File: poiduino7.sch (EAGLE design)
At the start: 20 parts, among them K1 TS-1109, Y1 16MHZ

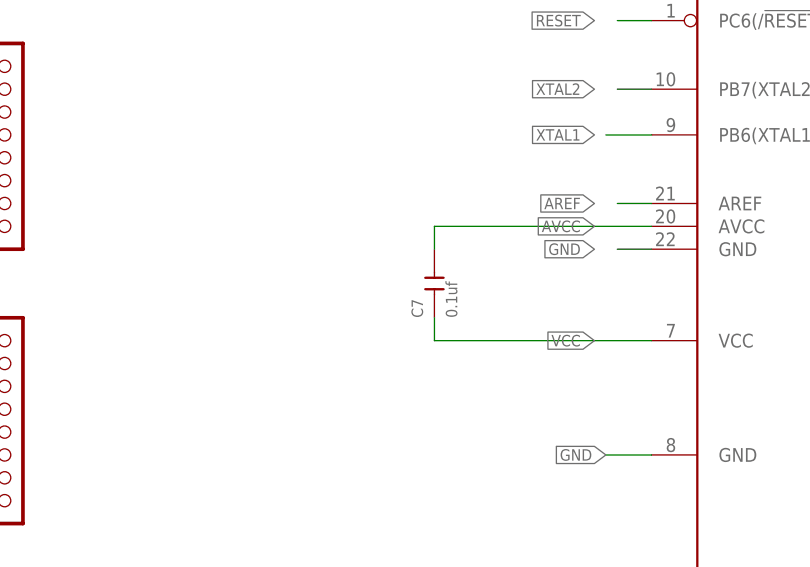
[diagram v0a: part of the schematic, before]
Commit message: new board
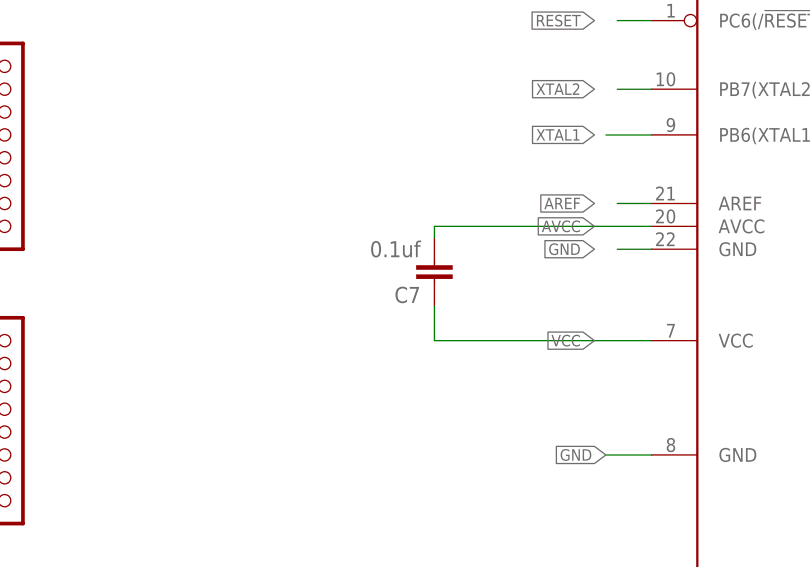
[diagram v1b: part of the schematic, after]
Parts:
- C7: device Seeed-Capacitor:DIP-CERAMIC-DISC-10NF-50V-Y5V(D4.0MM) -> capacitor-wima:C5/2.5
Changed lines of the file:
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@@
 <?xml version="1.0" encoding="utf-8"?>
 <!DOCTYPE eagle SYSTEM "eagle.dtd">
-<eagle version="7.7.0">
+<eagle version="9.0.0">
 <drawing>
 <settings>
 <setting alwaysvectorfont="no"/>
+<setting keepoldvectorfont="yes"/>
 <setting verticaltext="up"/>
 </settings>
-<grid distance="0.05" unitdist="inch" unit="inch" style="lines" multiple="1" display="yes" altdistance="0.001" altunitdist="inch" altunit="inch"/>
+<grid distance="0.1" unitdist="inch" unit="inch" style="lines" multiple="1" display="no" altdistance="0.01" altunitdist="inch" altunit="inch"/>
 <layers>
 <layer number="1" name="Top" color="4" fill="1" visible="no" active="no"/>
@@
 <part name="D1" library="Seeed-LED" deviceset="DIP-LED-GREEN-GREEN(2P-D3MM)" device="" value="CX-G302DC"/>
 <part name="D2" library="Seeed-LED" deviceset="DIP-LED-GREEN-GREEN(2P-D3MM)" device="" value="CX-G302DC"/>
-<part name="U1" library="Seeed-IC" deviceset="MCU-ATMEGA328P-PU(DIP28)" device=""/>
+<part name="U1" library="Seeed-IC" library_urn="urn:adsk.eagle:library:470" deviceset="MCU-ATMEGA328P-PU(DIP28)" device="" package3d_urn="urn:adsk.eagle:package:32652/1"/>
 <part name="Y1" library="Seeed-Crystal Oscillator" deviceset="DIP-CRYSTAL-16MHZ-18PF-30PPM-40R(HC49US)" device="" value="16MHZ"/>
 <part name="R1" library="Seeed-Resistor" deviceset="DIP-RES-10K-5%-1/4W(PR-D2.3XL6.5MM)" device="" value="10K"/>
@@
 <part name="SUPPLY7" library="supply2" deviceset="GND" device=""/>
 <part name="P+3" library="supply1" deviceset="VCC" device=""/>
-<part name="C7" library="Seeed-Capacitor" deviceset="DIP-CERAMIC-DISC-10NF-50V-Y5V(D4.0MM)" device="" value="0.1uf"/>
+<part name="C7" library="capacitor-wima" library_urn="urn:adsk.eagle:library:116" deviceset="C" device="5/2.5" package3d_urn="urn:adsk.eagle:package:5426/1" value="0.1uf"/>
 </parts>
 <sheets>
@@
 <instance part="SUPPLY7" gate="GND" x="77.47" y="81.28"/>
 <instance part="P+3" gate="VCC" x="77.47" y="109.22"/>
-<instance part="C7" gate="G$1" x="67.31" y="-16.51" rot="R90"/>
+<instance part="C7" gate="G$1" x="67.31" y="-16.51" rot="R180"/>
 </instances>
 <busses>
@@
 <label x="85.09" y="-10.16" size="1.27" layer="95" rot="R180" xref="yes"/>
 <pinref part="C7" gate="G$1" pin="2"/>
-<wire x1="67.31" y1="-12.7" x2="67.31" y2="-10.16" width="0.1524" layer="91"/>
+<wire x1="67.31" y1="-11.43" x2="67.31" y2="-10.16" width="0.1524" layer="91"/>
 <wire x1="91.44" y1="-10.16" x2="67.31" y2="-10.16" width="0.1524" layer="91"/>
 </segment>
@@
 <label x="85.09" y="-22.86" size="1.27" layer="95" rot="R180" xref="yes"/>
 <pinref part="C7" gate="G$1" pin="1"/>
-<wire x1="67.31" y1="-20.32" x2="67.31" y2="-22.86" width="0.1524" layer="91"/>
+<wire x1="67.31" y1="-19.05" x2="67.31" y2="-22.86" width="0.1524" layer="91"/>
 <wire x1="67.31" y1="-22.86" x2="91.44" y2="-22.86" width="0.1524" layer="91"/>
 </segment>
@@
 </schematic>
 </drawing>
+<compatibility>
+<note version="8.2" severity="warning">
+Since Version 8.2, EAGLE supports online libraries. The ids
+of those online libraries will not be understood (or retained)
+with this version.
+</note>
+<note version="8.3" severity="warning">
+Since Version 8.3, EAGLE supports URNs for individual library
+assets (packages, symbols, and devices). The URNs of those assets
+will not be understood (or retained) with this version.
+</note>
+<note version="8.3" severity="warning">
+Since Version 8.3, EAGLE supports the association of 3D packages
+with devices in libraries, schematics, and board files. Those 3D
+packages will not be understood (or retained) with this version.
+</note>
+</compatibility>
 </eagle>
